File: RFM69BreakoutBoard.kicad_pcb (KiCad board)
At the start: 2 copper layers, 26.2 x 25.8 mm, 0 parts

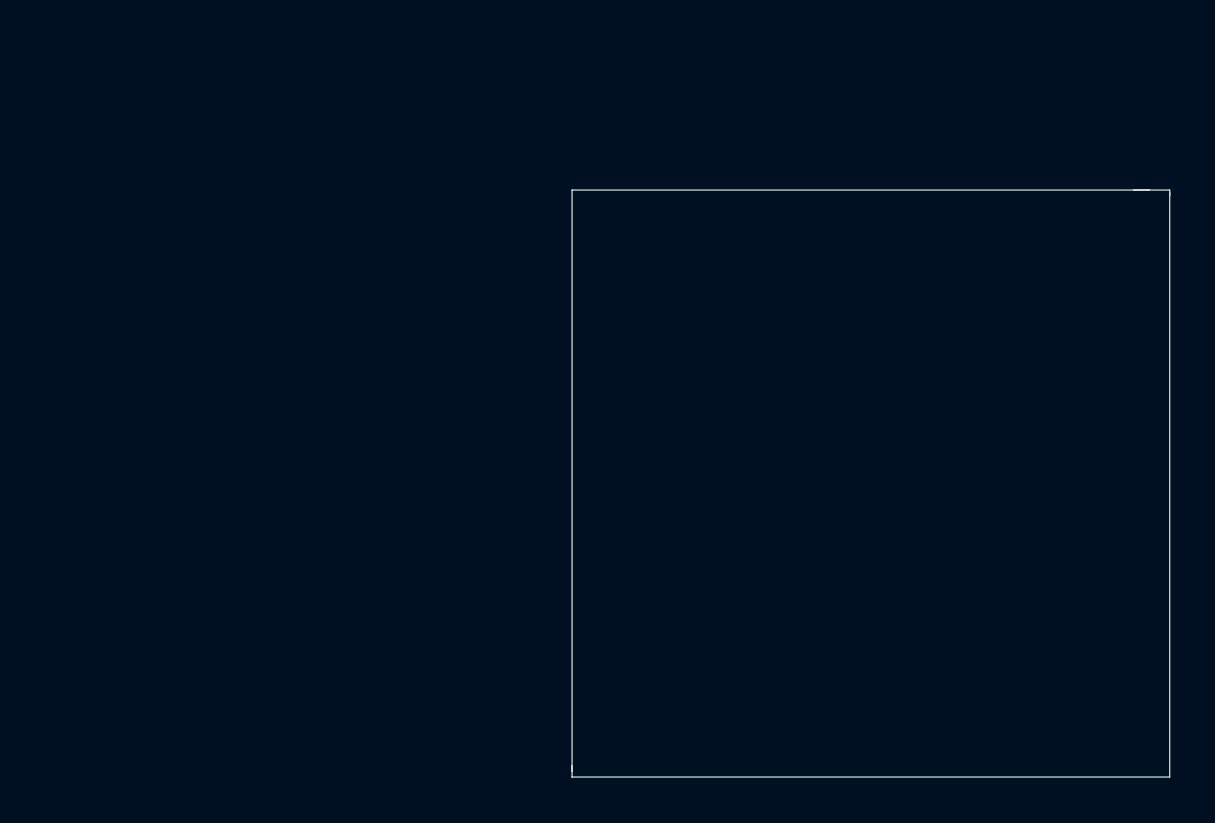
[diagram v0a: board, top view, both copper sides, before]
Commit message: first pass of trace
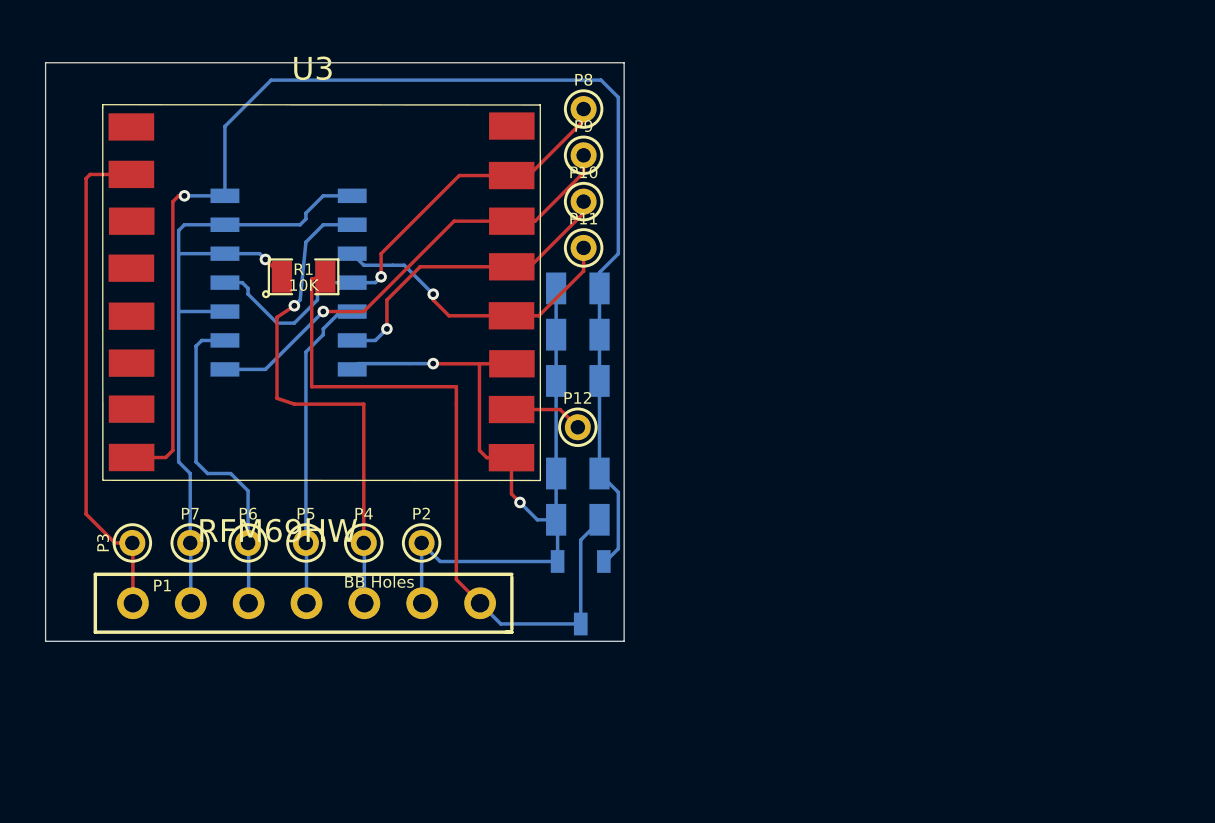
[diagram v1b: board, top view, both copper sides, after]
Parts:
- added C1: 1u, SM0805, B.Cu at (80.5, 153.4)
- added C2: 10u, SM0805, B.Cu at (80.5, 147.3)
- added C3: .1u, SM0805, B.Cu at (80.5, 151.4)
- added C4: 10u, SM0805, B.Cu at (80.5, 145.3)
- added C5: .1u, SM0805, B.Cu at (80.5, 143.3)
- added P1: BB Holes, 7_PINS, F.Cu at (67.3, 157.1)
- added P10: TST, PINTST, F.Cu at (80.8, 139.4)
- added P11: TST, PINTST, F.Cu at (80.8, 141.5)
- added P12: TST, PINTST, F.Cu at (80.5, 149.4)
- added P2: TST, PINTST, F.Cu at (73.7, 154.4)
- added P3: TST, PINTST, F.Cu at (61.0, 154.4)
- added P4: TST, PINTST, F.Cu at (71.1, 154.4)
- added P5: TST, PINTST, F.Cu at (68.6, 154.4)
- added P6: TST, PINTST, F.Cu at (66.0, 154.4)
- added P7: TST, PINTST, F.Cu at (63.5, 154.4)
- added P8: TST, PINTST, F.Cu at (80.8, 135.4)
- added P9: TST, PINTST, F.Cu at (80.8, 137.4)
- added R1: 10K, SM0805, F.Cu at (68.5, 142.7)
- added U1: MCP1703, SOT-23A, B.Cu at (79.2, 156.0)
- added U2: 74HCT123, so-14, B.Cu at (67.8, 143.0)
- added U3: RFM69HW, RFM69HW, F.Cu at (68.9, 144.4)
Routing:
- net +3.3V: track 0.00 -> 58.1 mm, vias 0 -> 1
- net GND: track 0.00 -> 37.5 mm, vias 0 -> 2
- net /CS_5V: track 0.00 -> 32.0 mm, vias 0 -> 1
- net +5V: track 0.00 -> 31.3 mm
- net /CLK_5V: track 0.00 -> 22.3 mm, vias 0 -> 1
- net /INT: track 0.00 -> 22.0 mm
- net /CS_3V3: track 0.00 -> 21.7 mm, vias 0 -> 1
- net /MOSI_3V3: track 0.00 -> 20.1 mm, vias 0 -> 1
- net /MOSI_5V: track 0.00 -> 14.2 mm
- net /MISO: track 0.00 -> 14.0 mm
- net /MISO_3V3: track 0.00 -> 13.7 mm, vias 0 -> 1
- net /CLK_3V3: track 0.00 -> 13.3 mm, vias 0 -> 1
- net /ANA: track 0.00 -> 3.23 mm
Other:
- board size 26.2 x 25.8 mm -> 25.4 x 25.4 mm
- net class Default: clearance 0.254 -> 0.1524; trace_width 0.254 -> 0.1524; via_dia 0.889 -> 0.508; via_drill 0.635 -> 0.3302
- rule trace_clearance: 0.254 -> 0.1524
- rule trace_min: 0.254 -> 0.1524
- rule via_min_drill: 0.508 -> 0.3302
- rule via_min_size: 0.889 -> 0.508
